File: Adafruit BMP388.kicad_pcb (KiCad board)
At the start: 2 copper layers, 15 x 11.2 mm, 8 parts, among them IC1 BMP388, J1 Conn_01x04_Male, U2 MIC5225-3.3

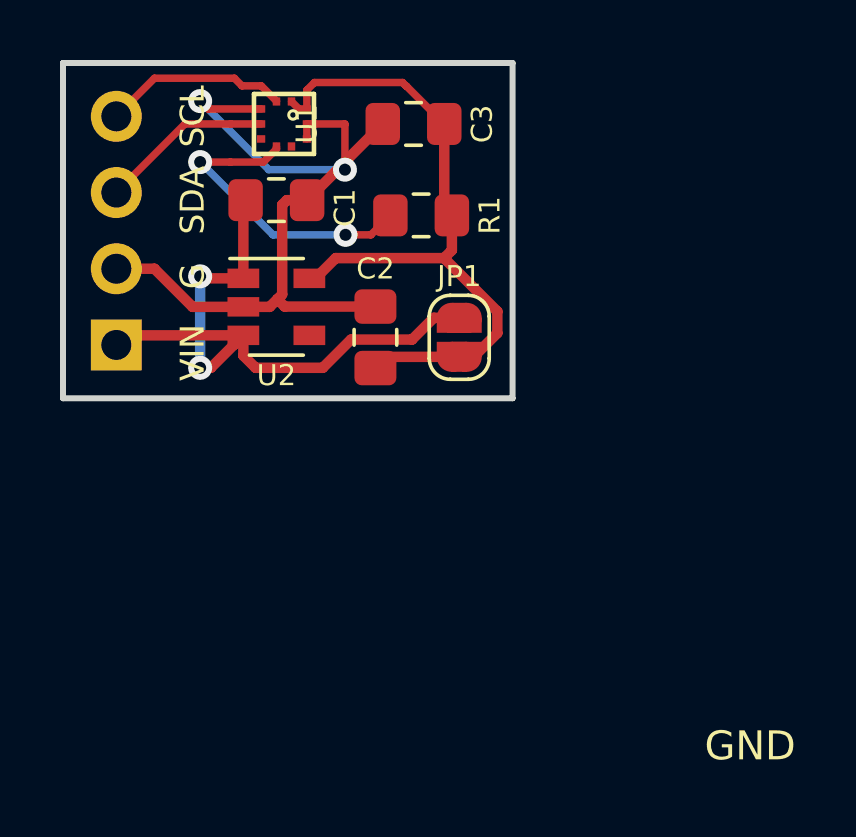
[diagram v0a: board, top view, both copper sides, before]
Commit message: update
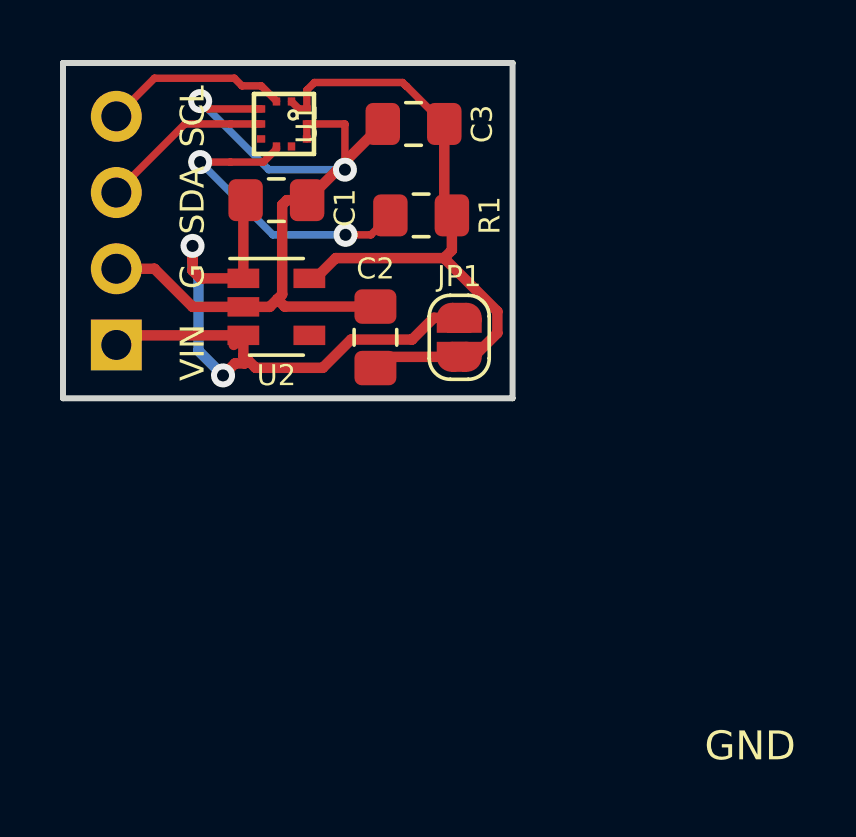
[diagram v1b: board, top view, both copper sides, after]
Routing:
- net VIN: track 22.9 -> 25.6 mm
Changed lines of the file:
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@@
     (thickness 1.6)
     (drawings 11)
-    (tracks 85)
+    (tracks 97)
     (zones 0)
     (modules 8)
@@
   (segment (start 127.932 91.007) (end 128.007 90.932) (width 0.35) (layer Top) (net 3) (status 30))
   (segment (start 127.932 93.538) (end 127.932 91.007) (width 0.35) (layer Top) (net 3) (status 30))
-  (segment (start 127.932 96.113) (end 128.339 96.52) (width 0.35) (layer Top) (net 3))
   (segment (start 127.932 95.438) (end 127.932 96.113) (width 0.35) (layer Top) (net 3) (status 10))
   (segment (start 127.932 93.538) (end 127.574 93.538) (width 0.25) (layer Top) (net 3) (status 30))
   (segment (start 124.018 95.438) (end 123.698 95.758) (width 0.35) (layer Top) (net 3) (status 30))
   (segment (start 127.932 95.438) (end 124.018 95.438) (width 0.35) (layer Top) (net 3) (status 30))
-  (via (at 126.492 96.52) (size 0.8) (drill 0.4) (layers Top Bottom) (net 3))
-  (segment (start 126.85 96.52) (end 127.932 95.438) (width 0.35) (layer Top) (net 3) (status 20))
-  (segment (start 126.492 96.52) (end 126.85 96.52) (width 0.35) (layer Top) (net 3))
+  (via (at 127.254 96.774) (size 0.8) (drill 0.4) (layers Top Bottom) (net 3))
   (segment (start 131.521012 95.57899) (end 130.580002 96.52) (width 0.35) (layer Top) (net 3))
   (segment (start 133.555418 95.57899) (end 131.521012 95.57899) (width 0.35) (layer Top) (net 3))
@@
   (segment (start 134.280408 94.854) (end 133.555418 95.57899) (width 0.35) (layer Top) (net 3))
   (segment (start 130.580002 96.52) (end 128.339 96.52) (width 0.35) (layer Top) (net 3))
-  (via (at 126.492 93.472) (size 0.8) (drill 0.4) (layers Top Bottom) (net 3))
+  (via (at 126.238 92.456) (size 0.8) (drill 0.4) (layers Top Bottom) (net 3))
   (segment (start 127.932 93.538) (end 126.558 93.538) (width 0.35) (layer Top) (net 3))
   (segment (start 126.558 93.538) (end 126.492 93.472) (width 0.35) (layer Top) (net 3))
-  (segment (start 126.492 93.472) (end 126.492 96.52) (width 0.35) (layer Bottom) (net 3))
+  (segment (start 126.500315 93.538) (end 126.238 93.275685) (width 0.35) (layer Top) (net 3))
+  (segment (start 126.558 93.538) (end 126.500315 93.538) (width 0.35) (layer Top) (net 3))
+  (segment (start 126.434315 93.472) (end 126.492 93.472) (width 0.35) (layer Bottom) (net 3))
+  (segment (start 126.238 93.275685) (end 126.434315 93.472) (width 0.35) (layer Bottom) (net 3))
+  (segment (start 126.238 92.71) (end 126.238 93.275685) (width 0.35) (layer Bottom) (net 3))
+  (segment (start 126.434315 95.954315) (end 127.254 96.774) (width 0.35) (layer Bottom) (net 3))
+  (segment (start 126.434315 93.472) (end 126.434315 95.954315) (width 0.35) (layer Bottom) (net 3))
+  (segment (start 127.976999 96.374001) (end 128.085 96.266) (width 0.35) (layer Top) (net 3))
+  (segment (start 127.653999 96.374001) (end 127.976999 96.374001) (width 0.35) (layer Top) (net 3))
+  (segment (start 127.932 96.113) (end 128.085 96.266) (width 0.35) (layer Top) (net 3))
+  (segment (start 127.254 96.774) (end 127.653999 96.374001) (width 0.35) (layer Top) (net 3))
+  (segment (start 128.085 96.266) (end 128.339 96.52) (width 0.35) (layer Top) (net 3))
+  (segment (start 126.238 92.964) (end 126.238 92.456) (width 0.35) (layer Top) (net 3))
+  (segment (start 126.238 92.964) (end 126.238 92.71) (width 0.35) (layer Top) (net 3))
+  (segment (start 126.238 93.275685) (end 126.238 92.964) (width 0.35) (layer Top) (net 3))
+  (segment (start 126.238 92.964) (end 126.238 92.456) (width 0.35) (layer Bottom) (net 3))
   (segment (start 127.6335 86.868) (end 124.968 86.868) (width 0.25) (layer Top) (net 4))
   (segment (start 124.968 86.868) (end 123.698 88.138) (width 0.25) (layer Top) (net 4) (status 20))
